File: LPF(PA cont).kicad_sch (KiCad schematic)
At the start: 2 parts, among them K1 G5V-1, K2 G5V-1

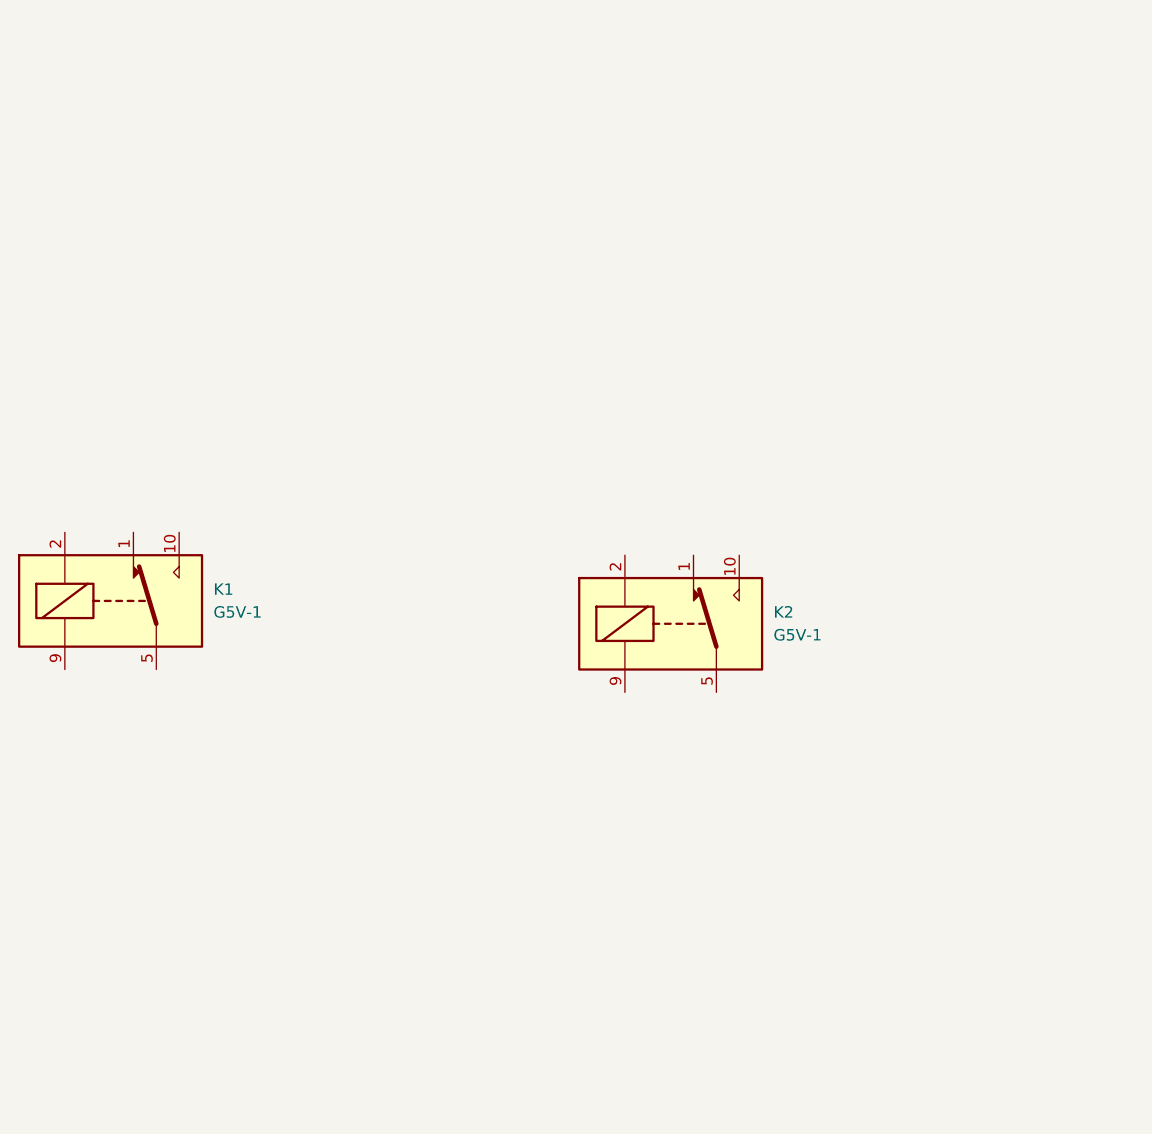
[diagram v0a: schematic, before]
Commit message: Logical Work
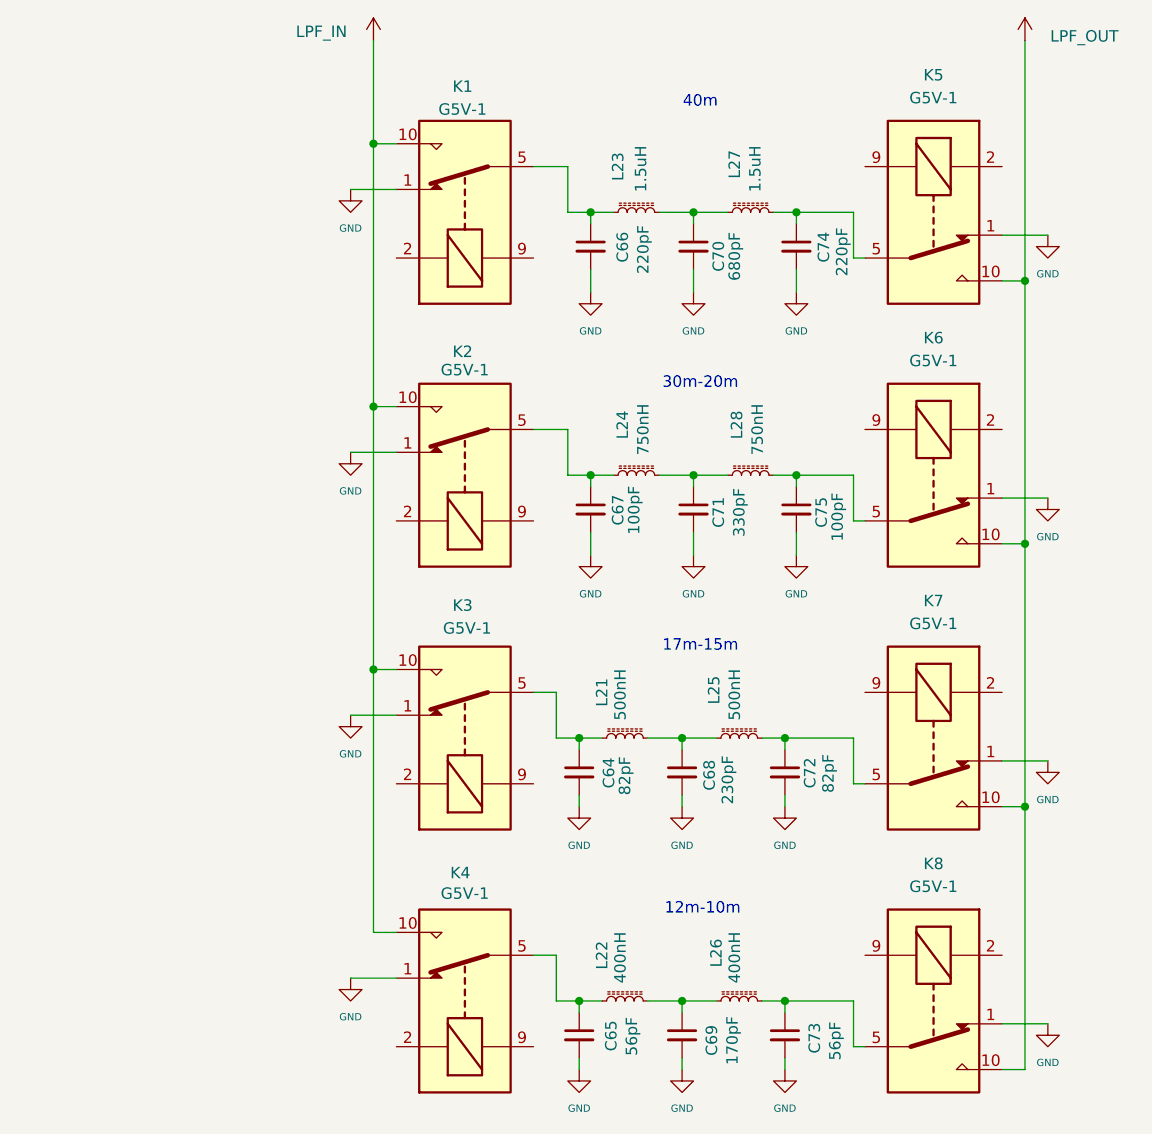
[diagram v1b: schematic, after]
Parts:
- added C64, C72: 82pF, symbol Device:C_Small
- added C65, C73: 56pF, symbol Device:C_Small
- added C66, C74: 220pF, symbol Device:C_Small
- added C67, C75: 100pF, symbol Device:C_Small
- added C68: 230pF, symbol Device:C_Small
- added C69: 170pF, symbol Device:C_Small
- added C70: 680pF, symbol Device:C_Small
- added C71: 330pF, symbol Device:C_Small
- added K3, K4, K5, K6, K7, K8: G5V-1, Relay_THT:Relay_SPDT_Omron_G5V-1, symbol Relay:G5V-1
- added L21, L25: 500nH, symbol Device:L_Ferrite_Small
- added L22, L26: 400nH, symbol Device:L_Ferrite_Small
- added L23, L27: 1.5uH, symbol Device:L_Ferrite_Small
- added L24, L28: 750nH, symbol Device:L_Ferrite_Small
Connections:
- net GND: now reaches K2.1
- net GND: now also K1.1, C64.2, C65.2, C66.2, C67.2, C68.2, C69.2, C70.2, C71.2, C72.2, C73.2, C74.2, C75.2, K3.1, K4.1, K5.1, K6.1, K7.1, K8.1
- net LPF_IN: now reaches K2.10
- net LPF_IN: now also K1.10, K3.10, K4.10
- net at K2.5, K2.6: now also C67.1, L24.1
- net at K1.5, K1.6: now also C66.1, L23.1
- new net: C75.1, K6.5, K6.6, L28.2
- new net: C74.1, K5.5, K5.6, L27.2
- new net: C71.1, L24.2, L28.1
- new net: C70.1, L23.2, L27.1
- new net: C69.1, L22.2, L26.1
- new net: C73.1, K8.5, K8.6, L26.2
- new net: C64.1, K3.5, K3.6, L21.1
- new net: C68.1, L21.2, L25.1
- new net: C72.1, K7.5, K7.6, L25.2
- new net: C65.1, K4.5, K4.6, L22.1
- new net LPF_OUT: K5.10, K6.10, K7.10, K8.10
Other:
- note added: "12m-10m"
- note added: "17m-15m"
- note added: "30m-20m"
- note added: "40m"
